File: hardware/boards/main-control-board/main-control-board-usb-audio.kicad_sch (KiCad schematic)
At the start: 8 parts, among them J1 Conn_01x02_Pin_Speaker, U3 MAX98357AETE+T

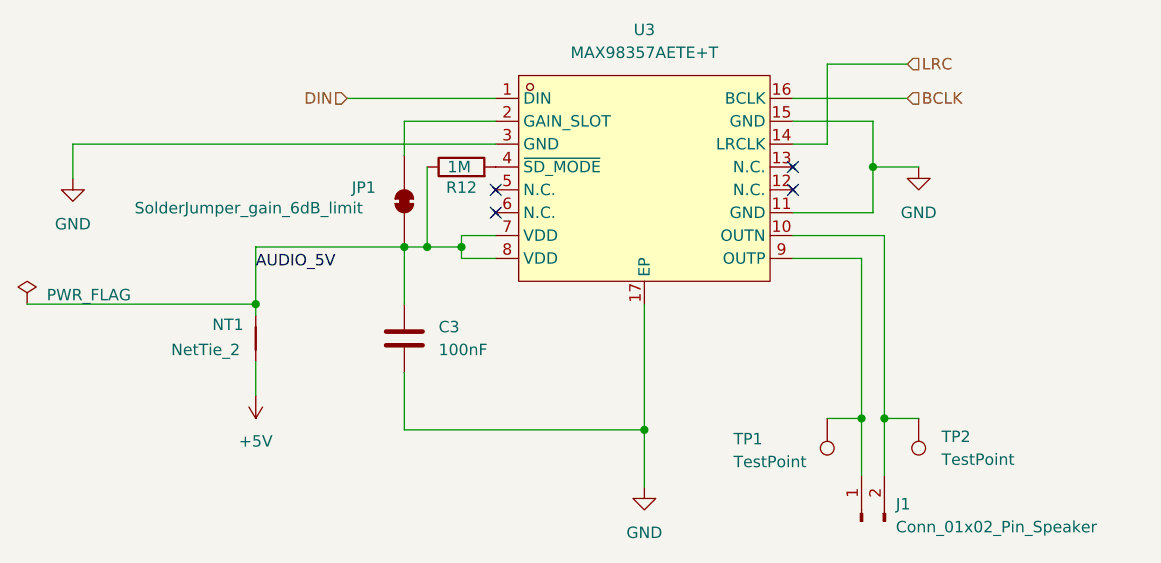
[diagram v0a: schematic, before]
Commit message: pre-fab improvements
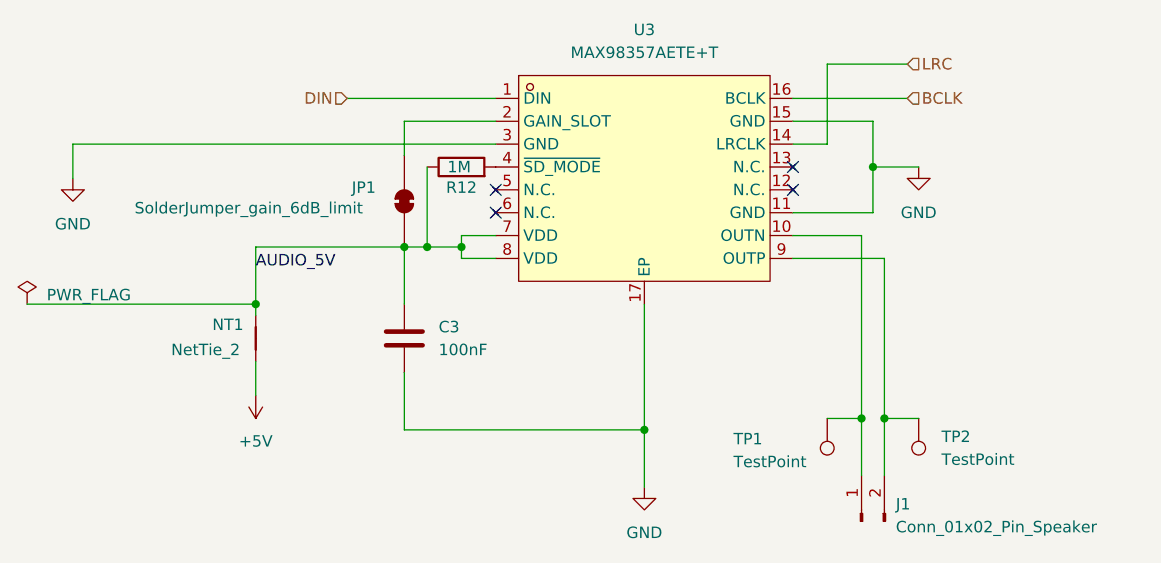
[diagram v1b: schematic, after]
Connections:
- net at J1.2 (Pin_2), TP2.1: now also U3.9 (OUTP); no longer U3.10 (OUTN)
- net at J1.1 (Pin_1), TP1.1: now also U3.10 (OUTN); no longer U3.9 (OUTP)
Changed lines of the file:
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@@
 	(paper "A4")
 	(junction
+		(at 115.57 68.58)
+		(diameter 0)
+		(color 0 0 0 0)
+	)
+	(junction
+		(at 166.37 87.63)
+		(diameter 0)
+		(color 0 0 0 0)
+	)
+	(junction
+		(at 99.06 74.93)
+		(diameter 0)
+		(color 0 0 0 0)
+	)
+	(junction
+		(at 167.64 59.69)
+		(diameter 0)
+		(color 0 0 0 0)
+	)
+	(junction
+		(at 142.24 88.9)
+		(diameter 0)
+		(color 0 0 0 0)
+	)
+	(junction
 		(at 168.91 87.63)
-		(diameter 0)
-		(color 0 0 0 0)
-	)
-	(junction
-		(at 115.57 68.58)
-		(diameter 0)
-		(color 0 0 0 0)
-	)
-	(junction
-		(at 166.37 87.63)
-		(diameter 0)
-		(color 0 0 0 0)
-	)
-	(junction
-		(at 99.06 74.93)
-		(diameter 0)
-		(color 0 0 0 0)
-	)
-	(junction
-		(at 167.64 59.69)
-		(diameter 0)
-		(color 0 0 0 0)
-	)
-	(junction
-		(at 142.24 88.9)
 		(diameter 0)
 		(color 0 0 0 0)
@@
 	(wire
 		(pts
-			(xy 166.37 69.85) (xy 166.37 87.63)
+			(xy 166.37 67.31) (xy 166.37 87.63)
 		)
 		(stroke
@@
 	(wire
 		(pts
-			(xy 168.91 67.31) (xy 168.91 87.63)
-		)
-		(stroke
-			(width 0)
-			(type default)
-		)
-	)
-	(wire
-		(pts
 			(xy 162.56 57.15) (xy 158.75 57.15)
 		)
@@
 	(wire
 		(pts
-			(xy 158.75 69.85) (xy 166.37 69.85)
+			(xy 158.75 69.85) (xy 168.91 69.85)
 		)
 		(stroke
@@
 	(wire
 		(pts
-			(xy 158.75 67.31) (xy 168.91 67.31)
+			(xy 158.75 67.31) (xy 166.37 67.31)
 		)
 		(stroke
@@
 		)
 		(stroke
+			(width 0)
+			(type default)
+		)
+	)
+	(wire
+		(pts
+			(xy 168.91 69.85) (xy 168.91 87.63)
+		)
+		(stroke
